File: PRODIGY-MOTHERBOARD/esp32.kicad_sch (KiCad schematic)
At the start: 3 parts, among them J18 Bus_M.2_Socket_A, P2 USB_C_Plug

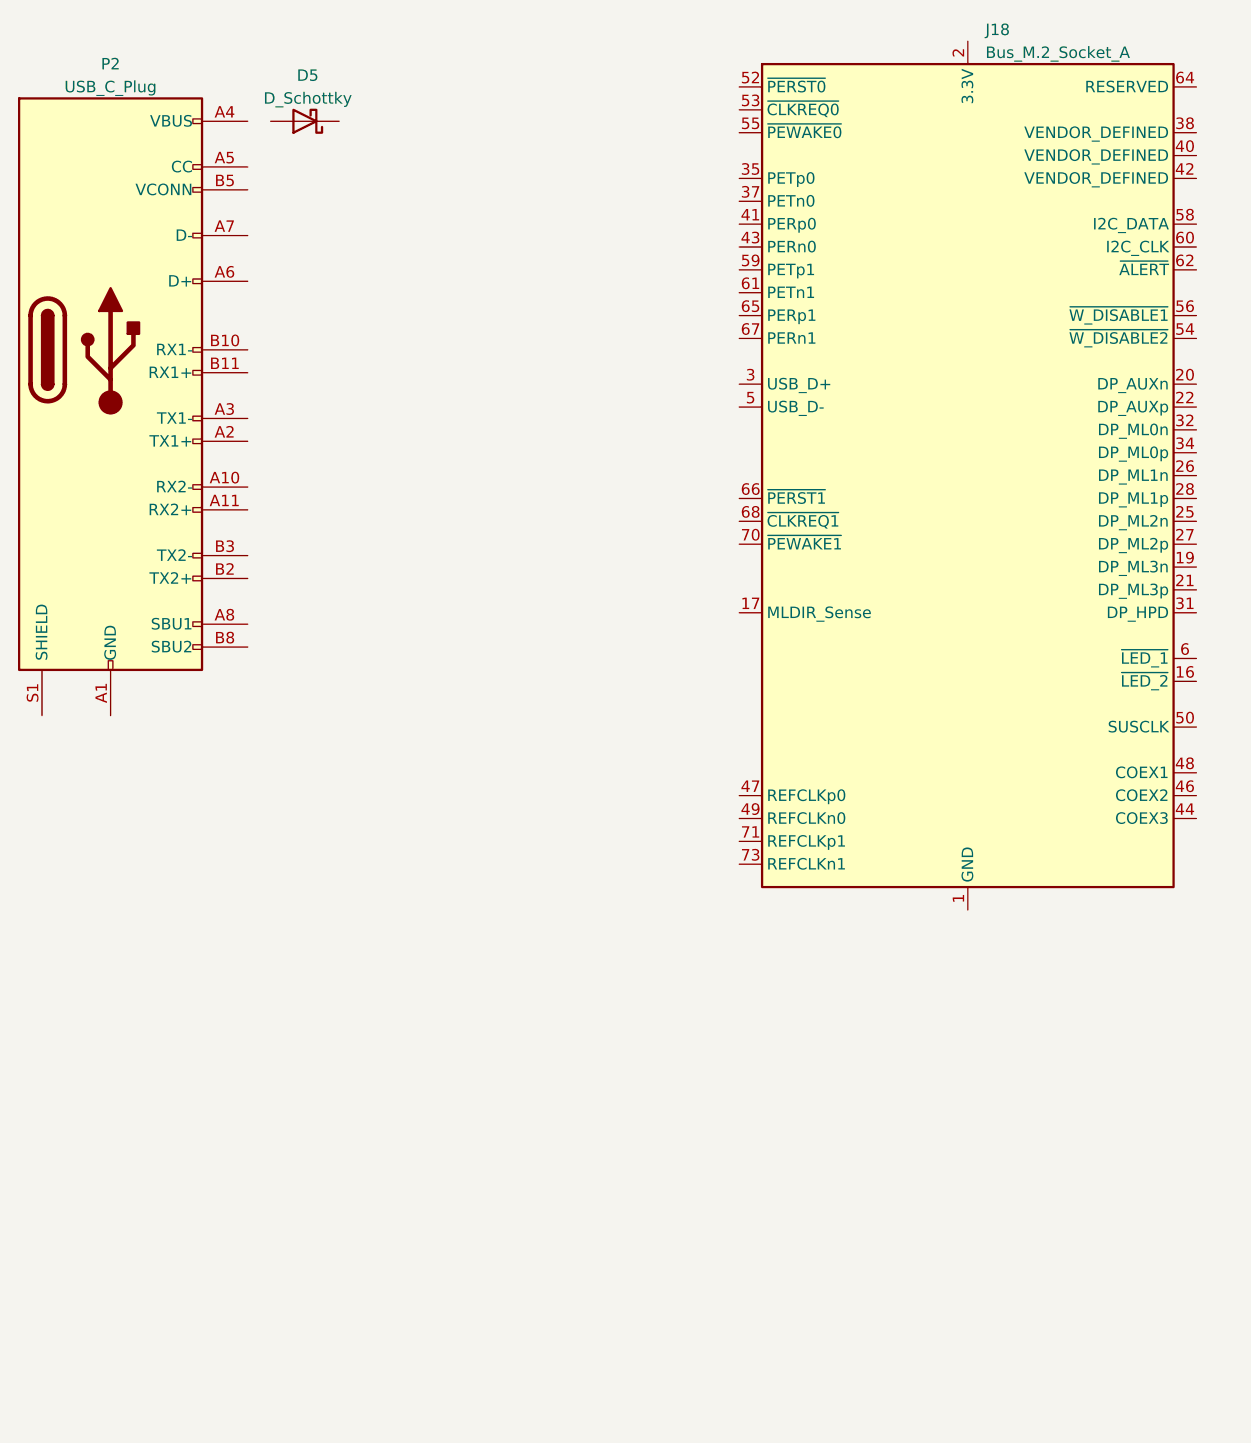
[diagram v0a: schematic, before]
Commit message: CAN schematic done
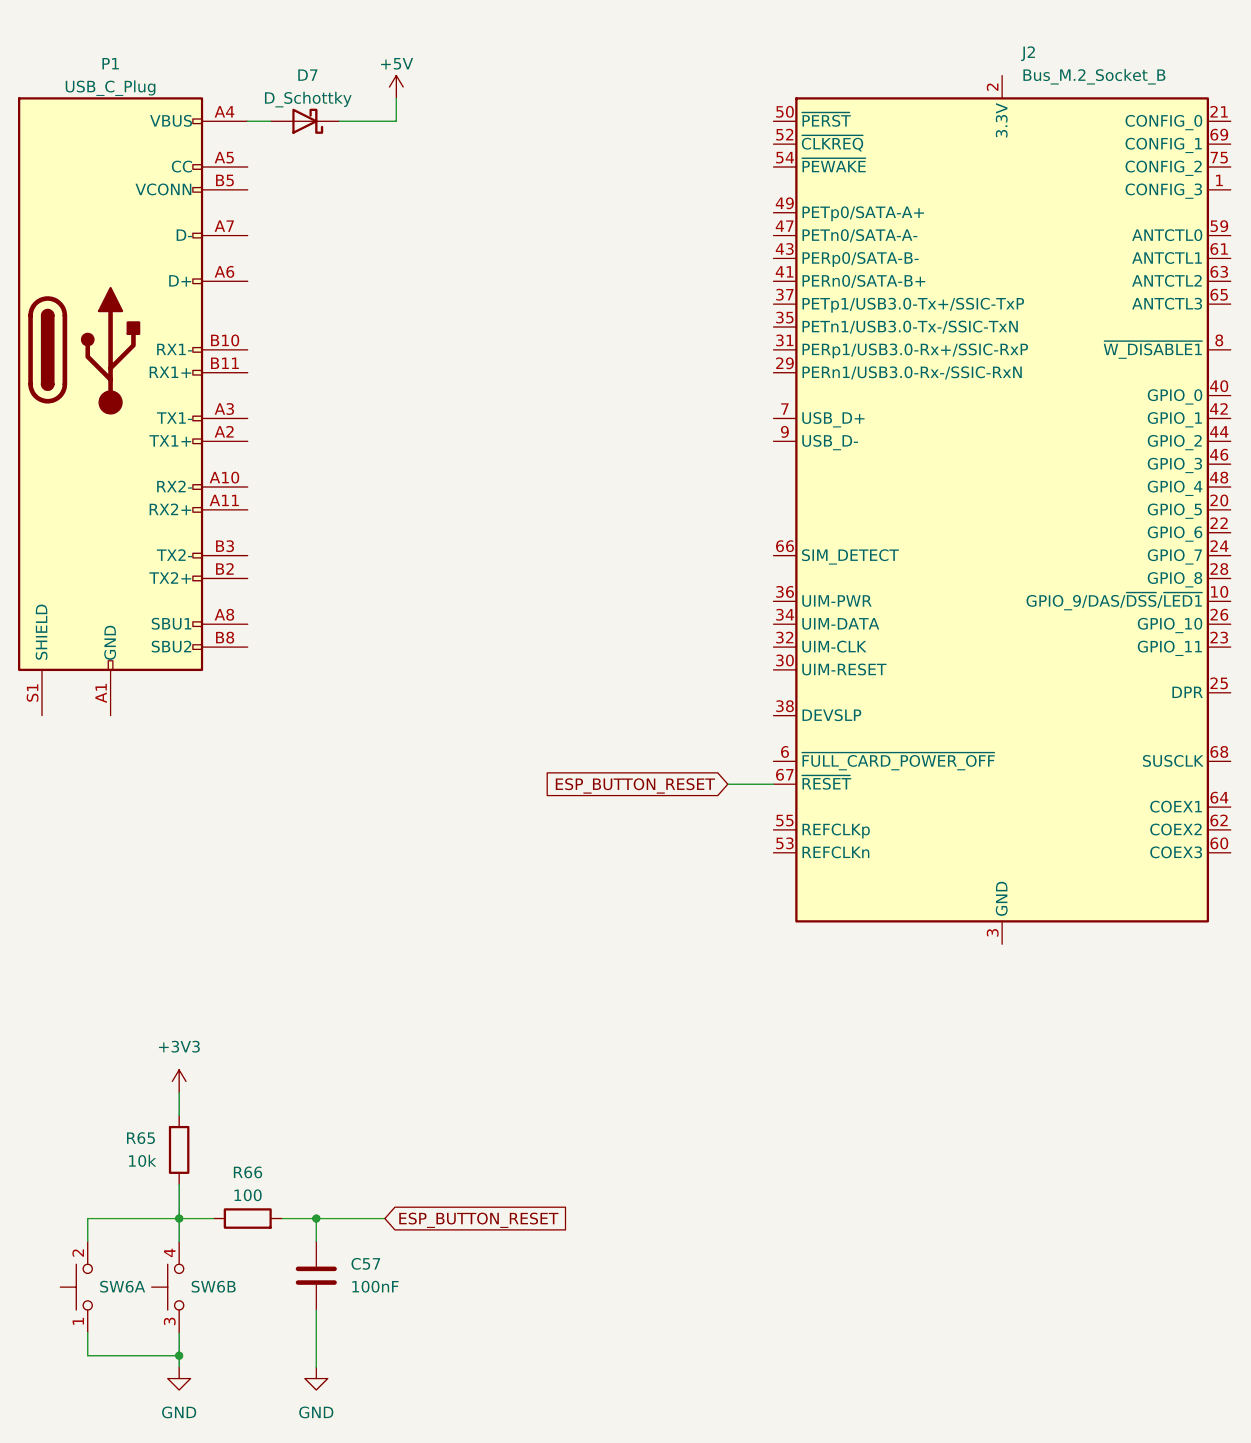
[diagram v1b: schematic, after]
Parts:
- removed J18: Bus_M.2_Socket_A, m.2_edge_connector_key_a:121992304, symbol Connector:Bus_M.2_Socket_A
- added C57: 100nF, symbol Device:C
- added J2: Bus_M.2_Socket_B, symbol Connector:Bus_M.2_Socket_B
- added R65: 10k, Resistor_SMD:R_0603_1608Metric, symbol Device:R
- added R66: 100, Resistor_SMD:R_0603_1608Metric, symbol Device:R
- added SW6: SW_Push_Dual_x2, symbol Switch:SW_Push_Dual_x2
- renumbered D5 to D7, P2 to P1
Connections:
- net +5V: now reaches D7.1 (K)
- net at D7.2 (A): now also P1.A4 (VBUS), P1.A9 (VBUS), P1.B4 (VBUS), P1.B9 (VBUS)
- new net: R65.1, R66.1, SW6.2 (D), SW6.4 (D)
- new net: J2.11 (GND), J2.27 (GND), J2.3 (GND), J2.33 (GND), J2.39 (GND), J2.45 (GND), J2.5 (GND), J2.51 (GND), J2.57 (GND), J2.71 (GND), J2.73 (GND)
- new net: J2.2 (3.3V), J2.4 (3.3V), J2.70 (3.3V), J2.72 (3.3V), J2.74 (3.3V)
- new net +3V3: R65.2
- new net ESP_BUTTON_RESET: C57.1, J2.67 (~{RESET}), R66.2
- new net GND: C57.2, SW6.1 (C), SW6.3 (C)
